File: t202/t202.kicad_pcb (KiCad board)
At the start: 2 copper layers, 23 x 12.2 mm, 7 parts, among them J1 Conn_02x04_Counter_Clockwise, SW1 SW_Push, U1 ATtiny202-SS

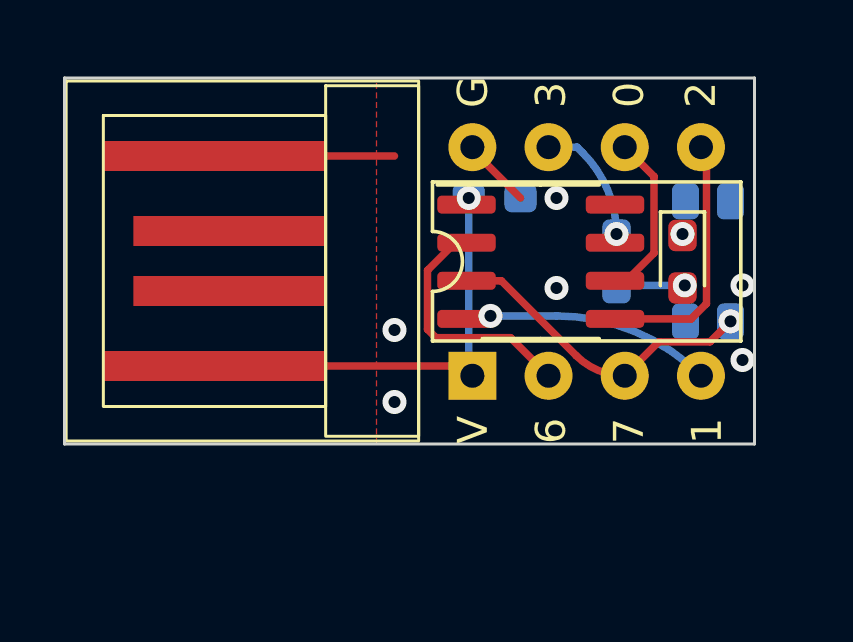
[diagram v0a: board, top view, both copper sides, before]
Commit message: -
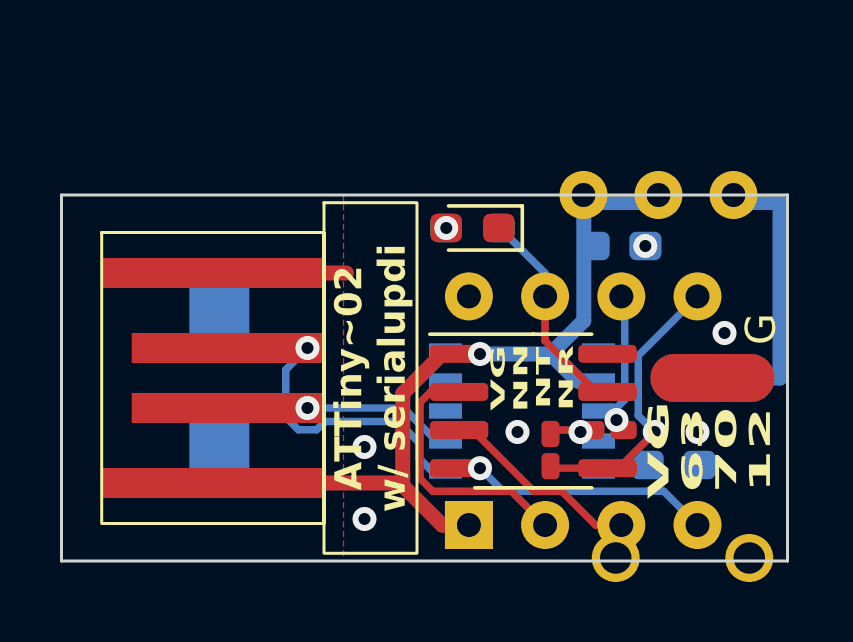
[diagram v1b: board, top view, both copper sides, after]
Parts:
- removed U2: ~, Library:PCB_USB_Conn
- added C2: 0u1, Capacitor_SMD:C_0603_1608Metric_Pad1.08x0.95mm_HandSolder, B.Cu at (120.3, 102.9)
- added C3: 1.5F, Library:ELDC_v, B.Cu at (123.7, 100.0)
- added J2: ~, Library:PCB_USB_Conn, F.Cu at (100.0, 100.0)
- added JP1: SolderJumper_2_Open, Library:sop_jumper, F.Cu at (116.2, 102.4)
- added SW2: SW_SPDT, Library:3pad_2.5_h, F.Cu at (119.8, 93.9)
- added U3: CH340K, Package_SO:SSOP-10_3.9x4.9mm_P1.00mm, B.Cu at (115.2, 101.1)
- C1: value C -> 0u1
- SW1: footprint Library:THAF01-NC-R -> Library:TVAF06-A020B-R; moved to F.Cu
- moved SW1 9.92 mm to (120.6, 106.0), turned to 90 degrees
- moved D1 7.09 mm to (113.6, 95.0), turned to 180 degrees
- moved U1 4.98 mm to (115.6, 101.1)
- moved J1 4.98 mm to (113.5, 104.9)
- moved R1 4.93 mm to (113.6, 95.0), turned to 180 degrees
- moved C1 4.46 mm to (118.5, 95.6)
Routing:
- net +5V: track 15.3 -> 27.6 mm
- net Net-(SW2-C): track 0.00 -> 9.65 mm
- net Net-(J2-D+): track 0.00 -> 9.20 mm, vias 0 -> 1
- net GND: track 9.82 -> 4.46 mm, vias 7 -> 6
- net Net-(J2-D-): track 0.00 -> 5.06 mm, vias 0 -> 1
- net Net-(J1-Pin_3): track 11.1 -> 6.72 mm, vias 1 -> 0
- net Net-(J1-Pin_7): track 4.51 -> 7.18 mm, vias 1 -> 0
- net Net-(D1-A): track 2.42 -> 0.00 mm
- net Net-(U3-V3): track 0.00 -> 1.72 mm
- net Net-(J1-Pin_5): track 8.52 -> 9.57 mm, vias 0 -> 1
- net Net-(J1-Pin_6): track 5.62 -> 5.94 mm, vias 0 -> 2
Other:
- board size 23 x 12.2 mm -> 24.2 x 12.2 mm
- board text added: "ATTiny~02 w/ serialupdi"
- board text added: "VG 63 70 12"
- board text added: "VG NN NT NR"
- board text added: "Vbat"
- board text removed: "0"
- board text removed: "1"
- board text removed: "2"
- board text removed: "3"
- board text removed: "6"
- board text removed: "7"
- board text removed: "V"
